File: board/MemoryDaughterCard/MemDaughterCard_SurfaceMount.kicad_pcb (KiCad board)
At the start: 2 copper layers, 86.5 x 68.3 mm, 18 parts, among them IC1 HM628512LFP-7, IC2 HM628512LFP-7, IC3 HM628512LFP-7, IC4 HM628512LFP-7, IC5 HM628512LFP-7, IC6 HM628512LFP-7, IC7 HM628512LFP-7, IC8 HM628512LFP-7, J1 Conn_01x32, J2 Conn_01x24, J3 E D C B A 9 8 7 6 5 4 3 2 1 0, J4 A B, U1 74LS139

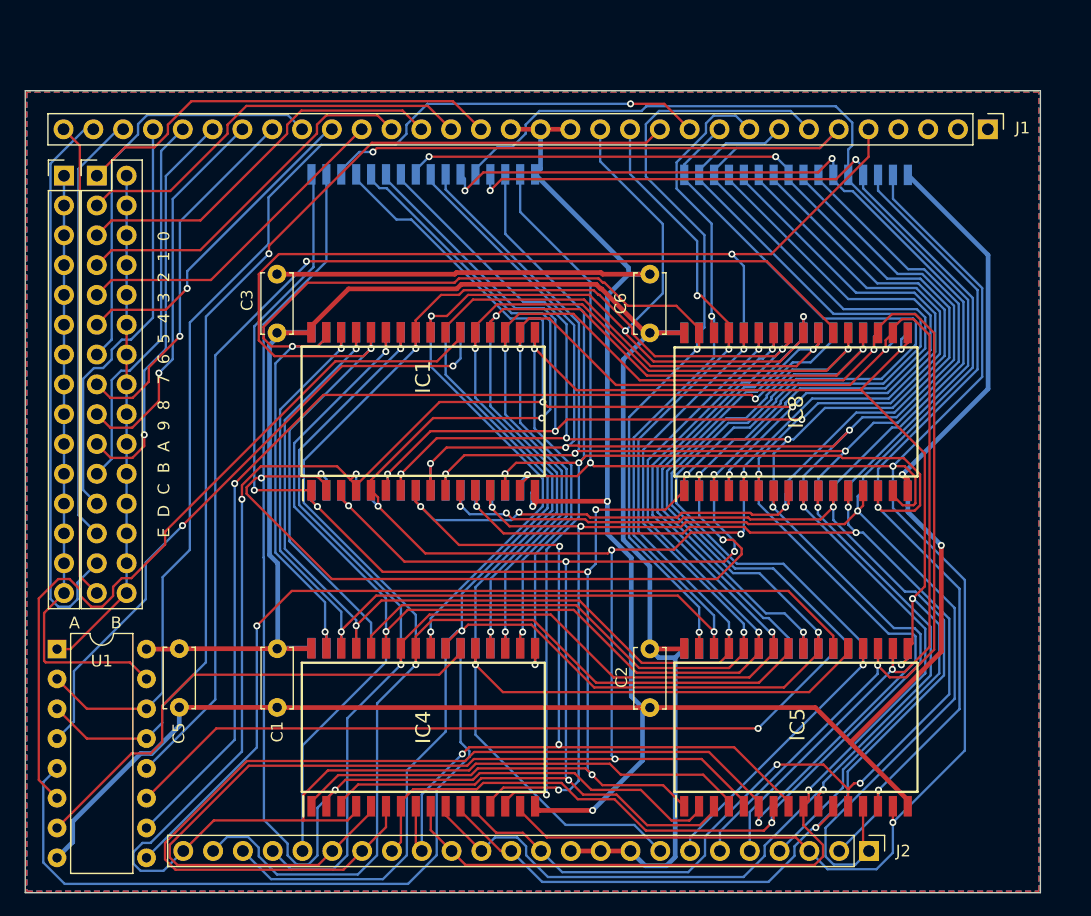
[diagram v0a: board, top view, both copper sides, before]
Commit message: Board V1.1G
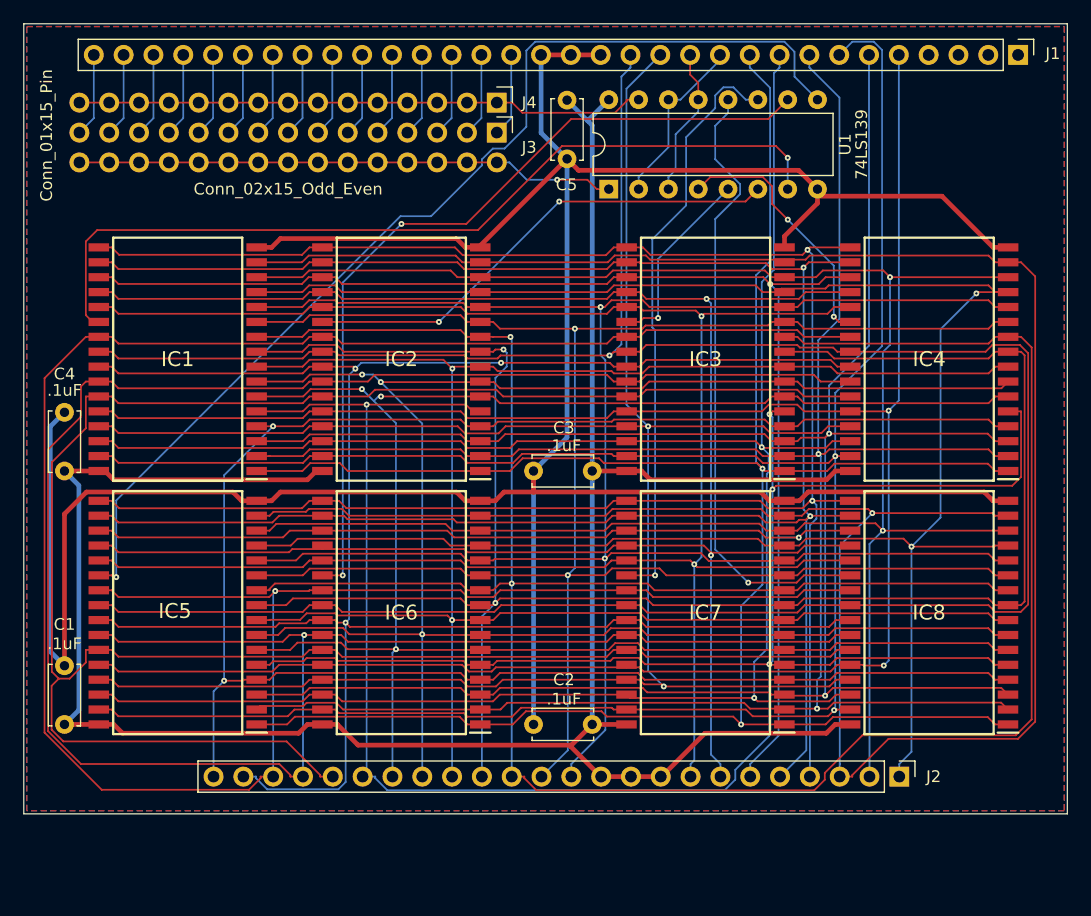
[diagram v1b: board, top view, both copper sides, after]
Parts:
- IC2, IC3, IC6, IC7: moved to F.Cu
- J3: value E D C B A 9 8 7 6 5 4 3 2 1 0 -> Conn_02x15_Odd_Even
- J4: value A B -> Conn_01x15_Pin
- moved U1 61.2 mm to (151.4, 103.0), turned to 90 degrees
- moved C5 57.2 mm to (147.9, 95.4)
- moved IC5 53.6 mm to (114.7, 139.1), turned to 180 degrees
- moved IC4 53.3 mm to (178.7, 117.5), turned to 180 degrees
- moved C4 51.2 mm to (105.1, 127.0)
- moved IC6 45.4 mm to (133.8, 139.1), turned to 180 degrees
- moved J4 37.4 mm to (141.9, 95.6), turned to -90 degrees
- moved J3 34.3 mm to (141.9, 98.2), turned to -90 degrees
- moved C3 29.3 mm to (150.0, 127.0), turned to 180 degrees
- moved IC3 25.7 mm to (159.7, 117.5), turned to 180 degrees
- moved IC1 21.4 mm to (114.7, 117.5), turned to 180 degrees
- moved IC8 20.5 mm to (178.7, 139.1), turned to 180 degrees
- moved C1 19.2 mm to (105.1, 148.6), turned to 90 degrees
- moved IC2 18.0 mm to (133.8, 117.5), turned to 180 degrees
- moved IC7 8.54 mm to (159.7, 139.1), turned to 180 degrees
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- renumbered C6 to C4
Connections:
- U1 pad 4: Net-(IC3-~{CS}) -> Net-(IC4-~{CS})
- U1 pad 5: Net-(IC2-~{CS}) -> Net-(IC3-~{CS})
- U1 pad 6: Net-(IC1-~{CS}) -> Net-(IC2-~{CS})
- U1 pad 7: Net-(IC4-~{CS}) -> Net-(IC1-~{CS})
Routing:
- net RAMB2: track 97.1 -> 14.9 mm, vias 1 -> 0
- net RAMB3: track 92.4 -> 12.8 mm, vias 1 -> 0
- net A6: track 238.5 -> 164.2 mm, vias 5 -> 3
- net !RWB: track 138.4 -> 210.2 mm, vias 5 -> 1
- net A12: track 231.9 -> 165.6 mm, vias 5 -> 2
- net A8: track 130.0 -> 192.8 mm, vias 4 -> 0
- net A9: track 139.2 -> 198.6 mm, vias 4 -> 1
- net RWB: track 128.0 -> 187.2 mm, vias 5 -> 2
- net RAMB0: track 128.6 -> 187.0 mm, vias 4 -> 2
- net +5v: track 150.8 -> 201.2 mm
- net D3: track 127.3 -> 176.6 mm, vias 5 -> 2
- net A2: track 181.4 -> 226.4 mm, vias 5 -> 2
- net D4: track 131.1 -> 175.6 mm, vias 4 -> 2
- net T3: track 231.6 -> 188.6 mm, vias 5 -> 2
- net Net-(IC8-~{CS}): track 96.5 -> 53.5 mm
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- added copper zone on F.Cu, net GND
- removed copper zone on B.Cu, net +5v
- removed copper zone on F.Cu, net +5v
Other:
- board size 86.5 x 68.3 mm -> 88.9 x 67.3 mm
